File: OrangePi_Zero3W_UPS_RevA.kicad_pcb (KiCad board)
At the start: 4 copper layers, 65 x 32 mm, 74 parts, among them J1 ORANGE_PI_ZERO_3W_HEADER, J2 BATTERY_1S_PROTECTED_NTC, J3 USB_C_POWER_INPUT, Q1 STL9P3LLH6, SW1 POWER / QON, U1 MAX17048G_T10, U2 BQ25895RTWR, U3 STUSB4500LQTR, U4 USBLC6-2SC6, U5 TPS61088RHLR, U6 TPS259470ARPWR

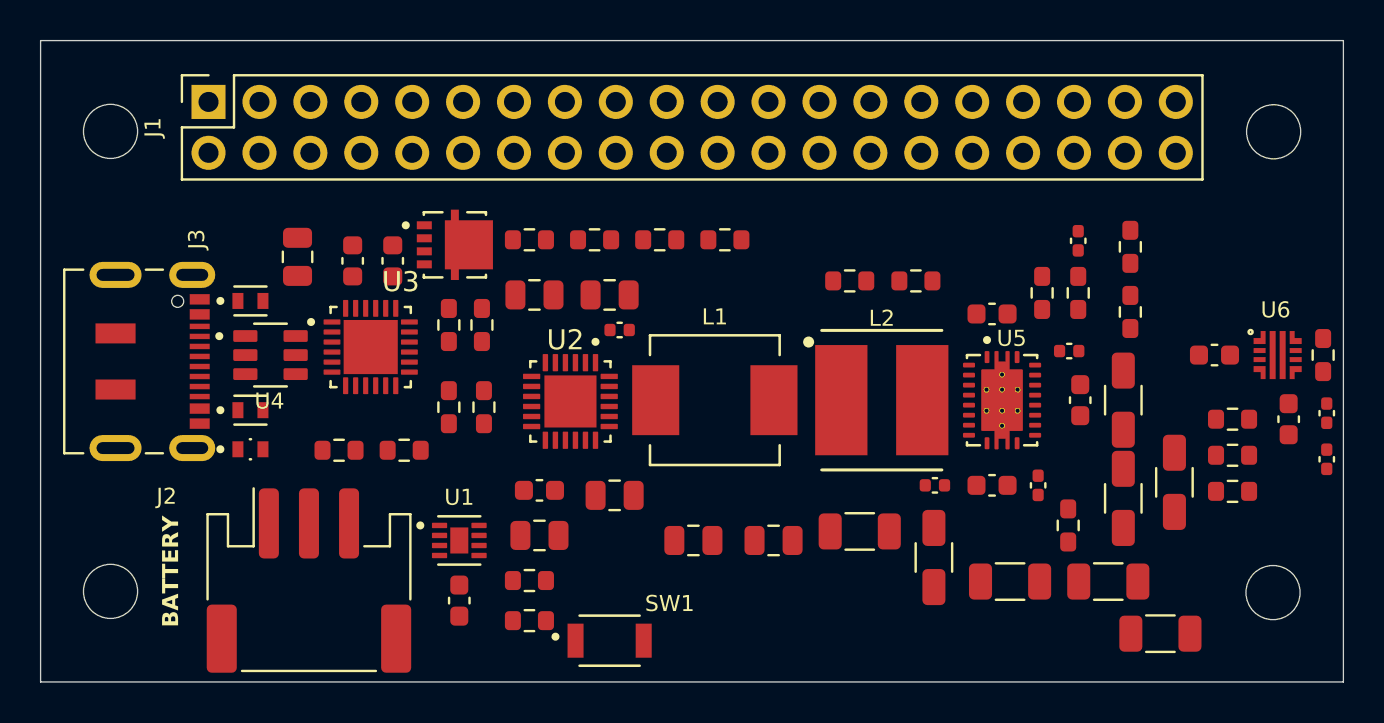
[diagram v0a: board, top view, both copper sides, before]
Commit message: Phase 6B.2B5: finalize placement clearance and assembly review
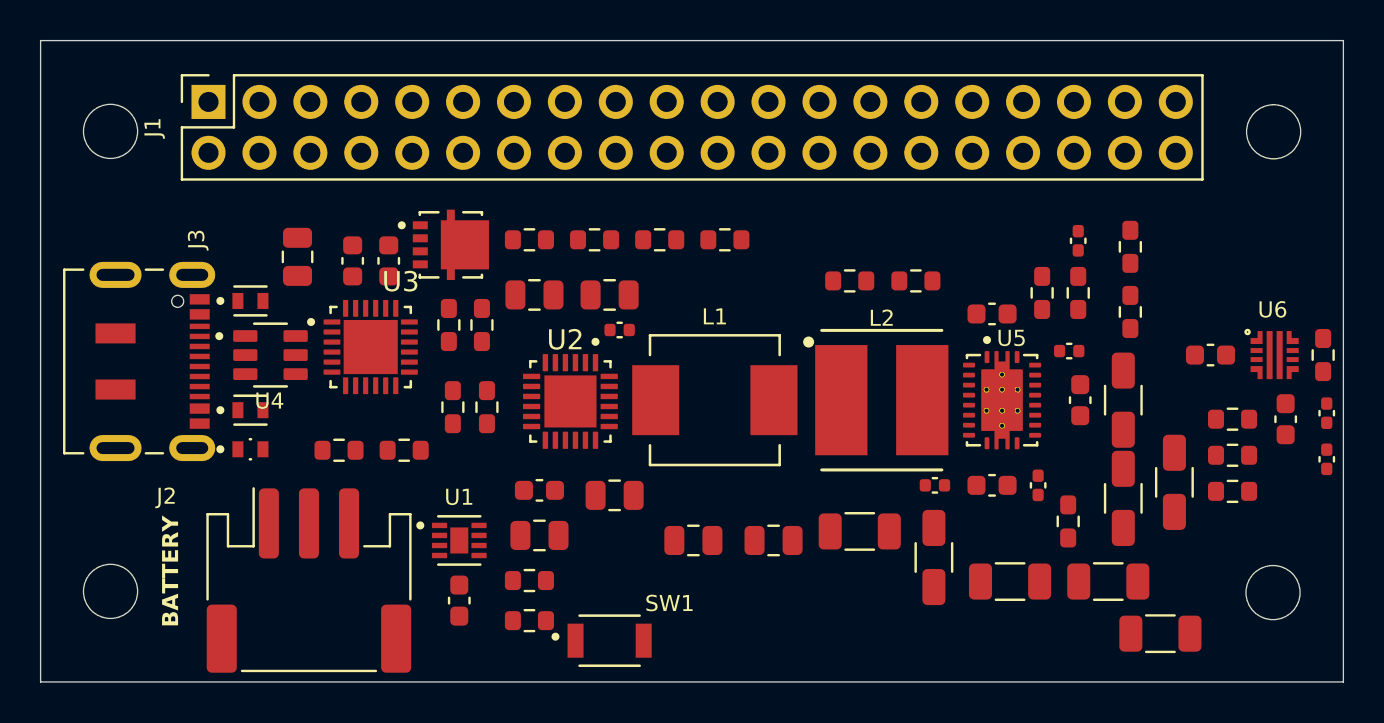
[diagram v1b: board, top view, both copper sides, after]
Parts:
- moved C26 0.20 mm to (114.0, 87.5)
- moved C8 0.20 mm to (73.0, 82.8)
- moved Q1 0.20 mm to (76.1, 82.0)
- moved R11 0.20 mm to (76.2, 90.1)
- moved R14 0.20 mm to (106.9, 95.8)
- moved C29 0.15 mm to (117.8, 90.7)
- moved R12 0.15 mm to (77.9, 90.1)
- moved U6 0.15 mm to (117.2, 87.5)
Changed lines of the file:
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@@
 	(footprint "Capacitor_SMD:C_0603_1608Metric"
 		(layer "F.Cu")
-		(at 73.200 82.800 90)
+		(at 73.000 82.800 90)
 		(descr "Capacitor SMD 0603 (1608 Metric), square (rectangular) end terminal, IPC-7351 nominal, (Body size source: IPC-SM-782 page 76, https://www.pcb-3d.com/wordpress/wp-content/uploads/ipc-sm-782a_amendment_1_and_2.pdf), generated with kicad-footprint-generator")
 		(tags "capacitor")
@@
 	(footprint "Resistor_SMD:R_0603_1608Metric"
 		(layer "F.Cu")
-		(at 76.000 90.100 90)
+		(at 76.200 90.100 90)
 		(descr "Resistor SMD 0603 (1608 Metric), square (rectangular) end terminal, IPC-7351 nominal, (Body size source: IPC-SM-782 page 72, https://www.pcb-3d.com/wordpress/wp-content/uploads/ipc-sm-782a_amendment_1_and_2.pdf), generated with kicad-footprint-generator")
 		(tags "resistor")
@@
 	(footprint "Resistor_SMD:R_0603_1608Metric"
 		(layer "F.Cu")
-		(at 77.750 90.100 90)
+		(at 77.900 90.100 90)
 		(descr "Resistor SMD 0603 (1608 Metric), square (rectangular) end terminal, IPC-7351 nominal, (Body size source: IPC-SM-782 page 72, https://www.pcb-3d.com/wordpress/wp-content/uploads/ipc-sm-782a_amendment_1_and_2.pdf), generated with kicad-footprint-generator")
 		(tags "resistor")
@@
 	(footprint "Resistor_SMD:R_0603_1608Metric"
 		(layer "F.Cu")
-		(at 106.900 96.000 -90)
+		(at 106.900 95.800 -90)
 		(descr "Resistor SMD 0603 (1608 Metric), square (rectangular) end terminal, IPC-7351 nominal, (Body size source: IPC-SM-782 page 72, https://www.pcb-3d.com/wordpress/wp-content/uploads/ipc-sm-782a_amendment_1_and_2.pdf), generated with kicad-footprint-generator")
 		(tags "resistor")
@@
 	(footprint "Capacitor_SMD:C_0603_1608Metric"
 		(layer "F.Cu")
-		(at 117.900 90.700 90)
+		(at 117.750 90.700 90)
 		(descr "Capacitor SMD 0603 (1608 Metric), square (rectangular) end terminal, IPC-7351 nominal, (Body size source: IPC-SM-782 page 76, https://www.pcb-3d.com/wordpress/wp-content/uploads/ipc-sm-782a_amendment_1_and_2.pdf), generated with kicad-footprint-generator")
 		(tags "capacitor")
@@
 	(footprint "STL9P3LLH6:TRANS_STL9P3LLH6"
 		(layer "F.Cu")
-		(at 76.300 82.000)
+		(at 76.100 82.000)
 		(property "Reference" "Q1"
 			(at 0 -2.45 0)
@@
 	(footprint "TPS25947_fixed:TPS259470ARPWR_RPW0010A"
 		(layer "F.Cu")
-		(at 117.350 87.500)
+		(at 117.200 87.500)
 		(descr "Texas Instruments RPW0010A VQFN-HR-10, 2.0x2.0mm, 0.45mm pitch; corner terminals use duplicate same-number pad primitives to form the recommended L-shaped lands")
 		(tags "TPS25947 RPW0010A VQFN-HR-10 eFuse")
@@
 	(footprint "Capacitor_SMD:C_0603_1608Metric"
 		(layer "F.Cu")
-		(at 114.200 87.500)
+		(at 114.000 87.500)
 		(descr "Capacitor SMD 0603 (1608 Metric), square (rectangular) end terminal, IPC-7351 nominal, (Body size source: IPC-SM-782 page 76, https://www.pcb-3d.com/wordpress/wp-content/uploads/ipc-sm-782a_amendment_1_and_2.pdf), generated with kicad-footprint-generator")
 		(tags "capacitor")
